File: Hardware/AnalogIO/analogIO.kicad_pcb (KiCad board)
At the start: 4 copper layers, 70 x 67.5 mm, 53 parts, among them J1 ANALOG INPUTS, J2 ANALOG OUTPUTS, J3 NUCLEO LEFT, J4 NUCLEO RIGHT, T1 AI0, T2 AI1, T3 AO0_OUT, T4 AO1_OUT, T5 AO0_BUFF, T6 AO1_BUFF, U1 LM358, U2 LM358, U3 LM358

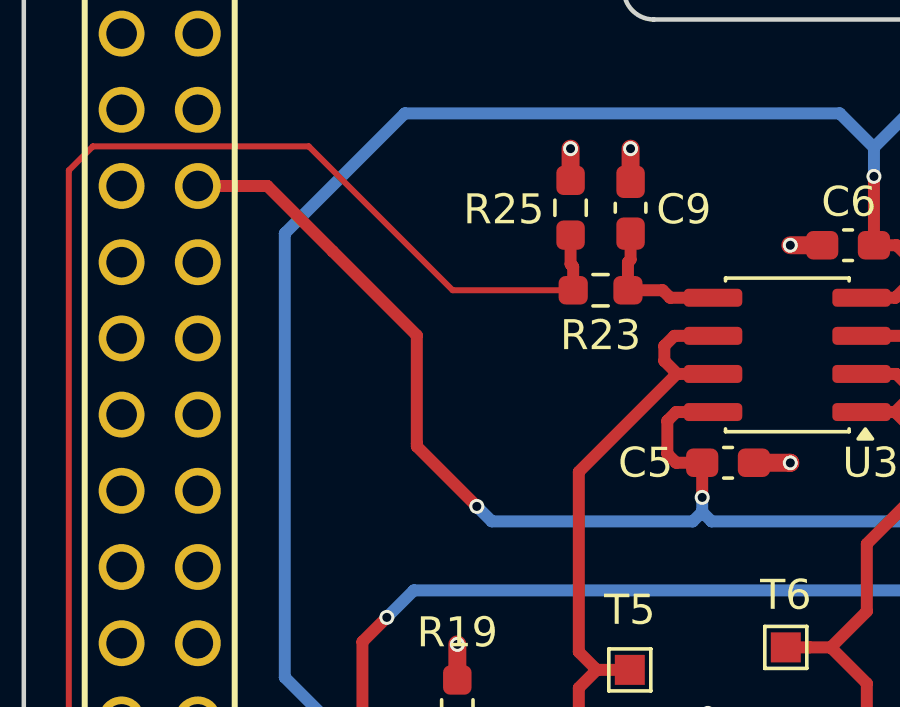
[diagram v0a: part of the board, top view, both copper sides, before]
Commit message: small adjustments and final revision
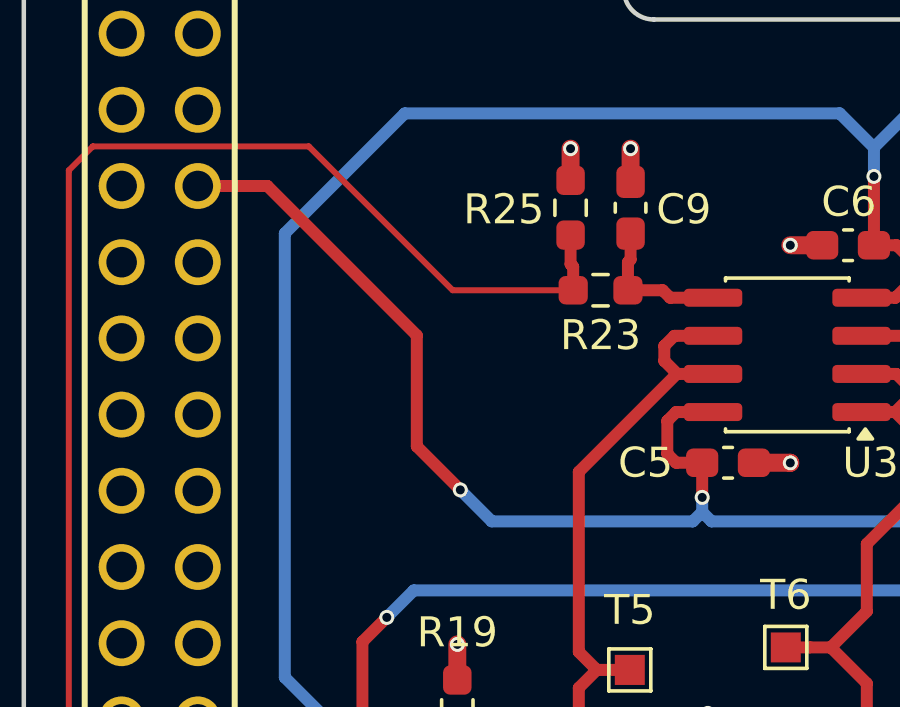
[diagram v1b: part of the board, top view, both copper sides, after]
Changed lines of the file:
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@@
 		(layer "Edge.Cuts")
+	)
+	(dimension
+		(type orthogonal)
+		(layer "Dwgs.User")
+		(pts
+			(xy 118.03 51.165) (xy 183.97 51.165)
+		)
+		(height -4.165)
+		(orientation 0)
+		(format
+			(prefix "")
+			(suffix "")
+			(units 3)
+			(units_format 1)
+			(precision 4)
+			(suppress_zeroes yes)
+		)
+		(style
+			(thickness 0.1)
+			(arrow_length 1.27)
+			(text_position_mode 1)
+			(arrow_direction outward)
+			(extension_height 0.58642)
+			(extension_offset 0.5)
+			(keep_text_aligned yes)
+		)
+		(gr_text "65.94 mm"
+			(at 151 47 0)
+			(layer "Dwgs.User")
+			(effects
+				(font
+					(size 0.8 0.8)
+					(thickness 0.1)
+				)
+			)
+		)
+	)
+	(dimension
+		(type orthogonal)
+		(layer "Dwgs.User")
+		(pts
+			(xy 116 112) (xy 186 112)
+		)
+		(height 14)
+		(orientation 0)
+		(format
+			(prefix "")
+			(suffix "")
+			(units 3)
+			(units_format 1)
+			(precision 4)
+			(suppress_zeroes yes)
+		)
+		(style
+			(thickness 0.1)
+			(arrow_length 1.27)
+			(text_position_mode 1)
+			(arrow_direction outward)
+			(extension_height 0.58642)
+			(extension_offset 0.5)
+			(keep_text_aligned yes)
+		)
+		(gr_text "70 mm"
+			(at 151 126 0)
+			(layer "Dwgs.User")
+			(effects
+				(font
+					(size 0.8 0.8)
+					(thickness 0.1)
+				)
+			)
+		)
+	)
+	(dimension
+		(type orthogonal)
+		(layer "Dwgs.User")
+		(pts
+			(xy 162 116) (xy 167 48.5)
+		)
+		(height 34)
+		(orientation 1)
+		(format
+			(prefix "")
+			(suffix "")
+			(units 3)
+			(units_format 1)
+			(precision 4)
+			(suppress_zeroes yes)
+		)
+		(style
+			(thickness 0.1)
+			(arrow_length 1.27)
+			(text_position_mode 1)
+			(arrow_direction outward)
+			(extension_height 0.58642)
+			(extension_offset 0.5)
+			(keep_text_aligned yes)
+		)
+		(gr_text "67.5 mm"
+			(at 196 82.25 90)
+			(layer "Dwgs.User")
+			(effects
+				(font
+					(size 0.8 0.8)
+					(thickness 0.1)
+				)
+			)
+		)
 	)
 	(segment
@@
 	)
 	(segment
-		(start 121.8 62.72)
-		(end 124.12 62.72)
-		(width 0.4)
-		(layer "F.Cu")
-		(net 31)
-	)
-	(segment
 		(start 170.7 93.4)
 		(end 170.44625 93.14625)
@@
 	)
 	(segment
-		(start 129.1 71.3)
-		(end 129.1 71.4)
+		(start 129.1 71.4)
+		(end 129.1 67.7)
 		(width 0.4)
 		(layer "F.Cu")
@@
 	)
 	(segment
-		(start 124.12 62.72)
-		(end 126.3 64.9)
-		(width 0.4)
-		(layer "F.Cu")
-		(net 31)
-	)
-	(segment
 		(start 138.6125 73.1)
 		(end 138.6125 71.945)
@@
 	)
 	(segment
-		(start 129.1 71.4)
-		(end 131.1 73.4)
+		(start 130.55 72.85)
+		(end 129.1 71.4)
 		(width 0.4)
 		(layer "F.Cu")
@@
 	)
 	(segment
-		(start 129.1 67.7)
-		(end 129.1 71.3)
-		(width 0.4)
-		(layer "F.Cu")
-		(net 31)
-	)
-	(segment
 		(start 134.7 87.95)
 		(end 134.7 88.95)
@@
 	)
 	(segment
-		(start 126.3 64.9)
-		(end 129.1 67.7)
-		(width 0.4)
-		(layer "F.Cu")
-		(net 31)
-	)
-	(segment
 		(start 135.165 89.415)
 		(end 135.9125 89.415)
@@
 	)
 	(segment
+		(start 124.12 62.72)
+		(end 121.8 62.72)
+		(width 0.4)
+		(layer "F.Cu")
+		(net 31)
+	)
+	(segment
+		(start 129.1 67.7)
+		(end 124.12 62.72)
+		(width 0.4)
+		(layer "F.Cu")
+		(net 31)
+	)
+	(segment
 		(start 136.2 90.6)
 		(end 135.9125 90.3125)
@@
 	)
 	(via
-		(at 131.1 73.4)
+		(at 130.55 72.85)
 		(size 0.5)
 		(drill 0.3)
@@
 	(segment
 		(start 138.3 73.9)
-		(end 131.6 73.9)
+		(end 138.6125 73.5875)
 		(width 0.4)
 		(layer "B.Cu")
@@
 	(segment
 		(start 131.6 73.9)
-		(end 131.1 73.4)
+		(end 138.3 73.9)
 		(width 0.4)
 		(layer "B.Cu")
@@
 	)
 	(segment
-		(start 138.6125 73.5875)
-		(end 138.3 73.9)
-		(width 0.4)
-		(layer "B.Cu")
+		(start 130.55 72.85)
+		(end 131.6 73.9)
+		(width 0.4)
+		(layer "B.Cu")
